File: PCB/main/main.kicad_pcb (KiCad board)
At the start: 2 copper layers, 4 parts, among them J1 Conn_01x33_Female, J2 Conn_01x33_Female, J3 Conn_01x33_Female, J4 Conn_01x33_Female

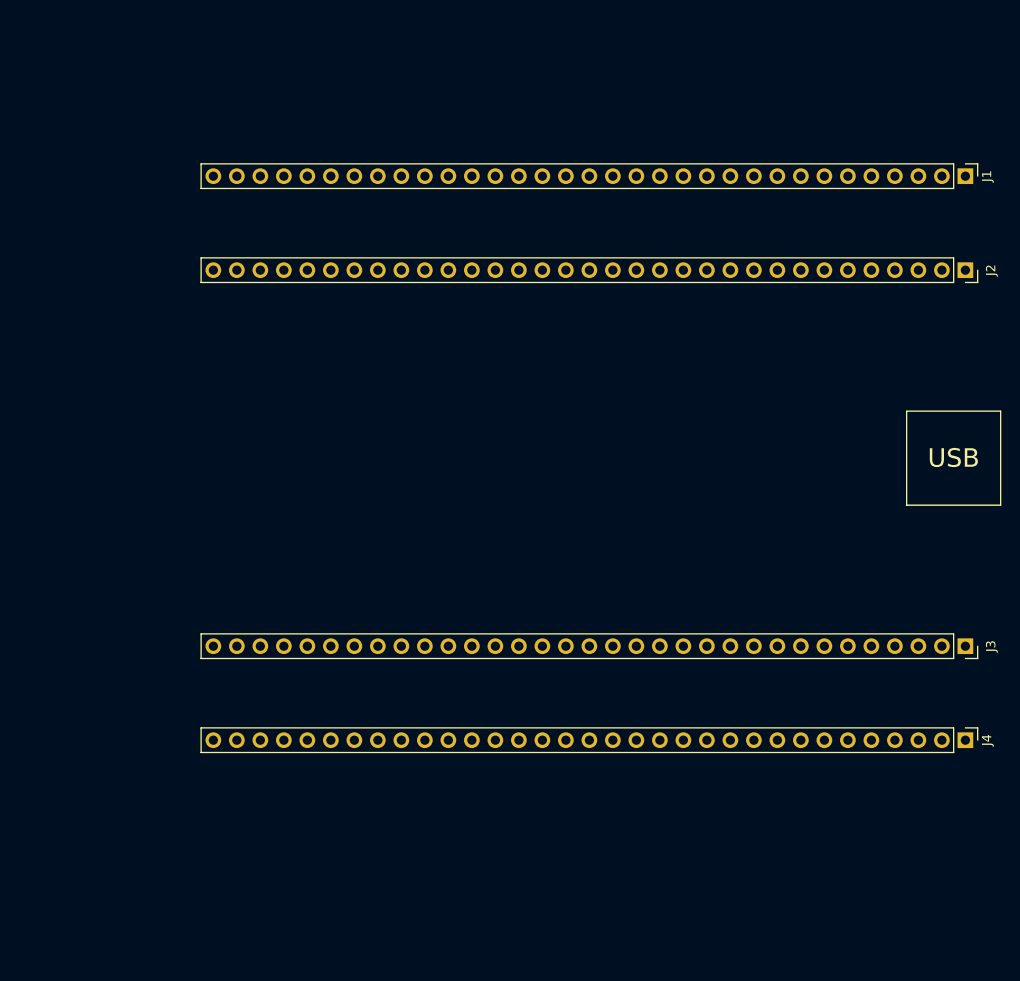
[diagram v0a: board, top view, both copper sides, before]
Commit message: NEW PCB ADDED
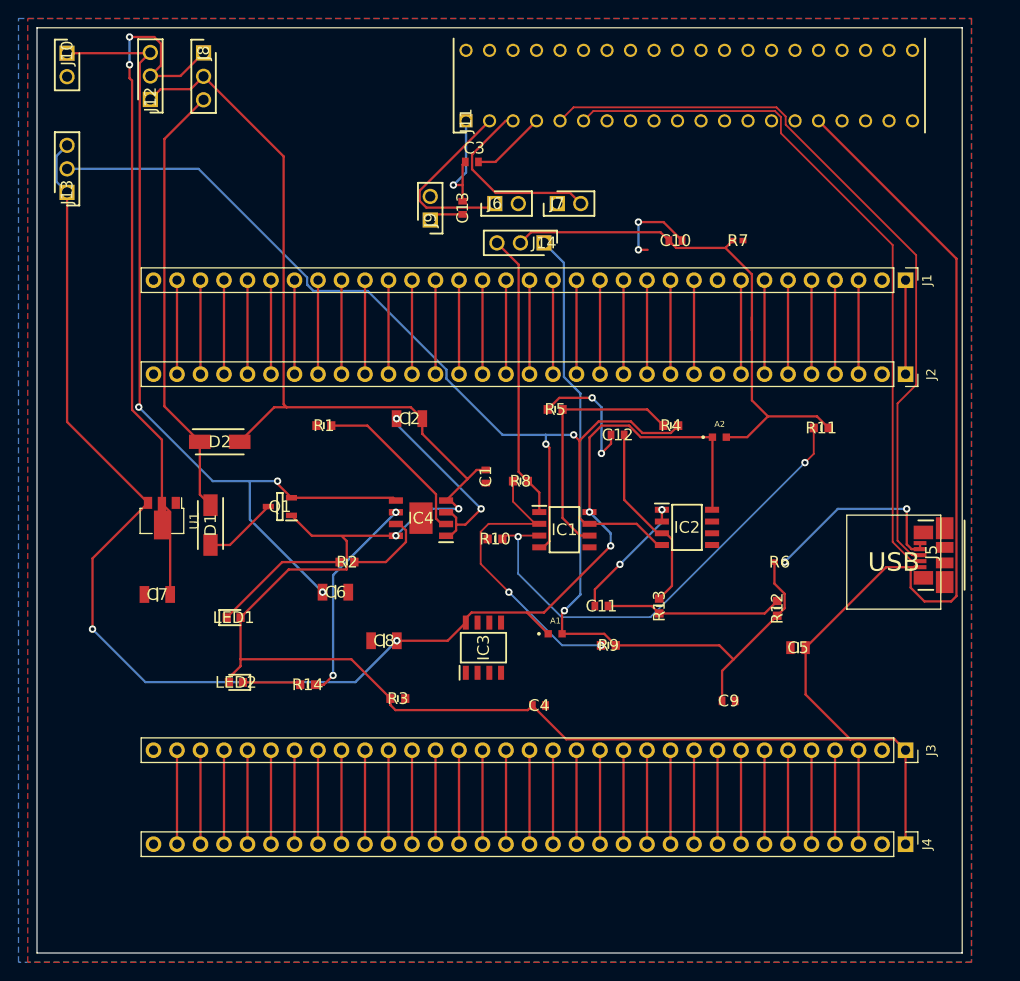
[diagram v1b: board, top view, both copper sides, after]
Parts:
- added A1: ALS-PT19-315C/L177/TR8, SamacSys_Parts:XDCR_ALS-PT19-315C_L177_TR8, F.Cu at (136.0, 115.5)
- added A2: ALS-PT19-315C/L177/TR8, SamacSys_Parts:XDCR_ALS-PT19-315C_L177_TR8, F.Cu at (153.8, 94.2)
- added C1: 10nF, SamacSys_Parts:CAPC1608X90N, F.Cu at (128.5, 98.5)
- added C10: CL10A105KB8NNNC, SamacSys_Parts:CAPC1608X90N, F.Cu at (149.0, 73.0)
- added C11: CL10A335KP8NNNC, SamacSys_Parts:CAPC1608X90N, F.Cu at (141.0, 112.5)
- added C12: CL10A335KP8NNNC, SamacSys_Parts:CAPC1608X90N, F.Cu at (142.8, 94.0)
- added C13: CC0603KRX7R9BB104, SamacSys_Parts:CAPC1608X90N, F.Cu at (126.0, 69.5)
- added C2: CL31A106KBHNNNE, SamacSys_Parts:CAPC3216X180N, F.Cu at (120.2, 92.2)
- added C3: 100nF, SamacSys_Parts:CAPC1608X90N, F.Cu at (127.0, 64.5)
- added C4: 100nF, SamacSys_Parts:CAPC1608X90N, F.Cu at (134.2, 123.2)
- added C5: CL21C101JBANNNC, SamacSys_Parts:CAPC2012X75N, F.Cu at (162.2, 117.0)
- added C6: CL31A106KBHNNNE, SamacSys_Parts:CAPC3216X180N, F.Cu at (112.2, 111.0)
- added C7: CL31A106KBHNNNE, SamacSys_Parts:CAPC3216X180N, F.Cu at (93.0, 111.2)
- added C8: CL31A106KBHNNNE, SamacSys_Parts:CAPC3216X180N, F.Cu at (117.5, 116.2)
- added C9: CL10A105KB8NNNC, SamacSys_Parts:CAPC1608X90N, F.Cu at (154.8, 122.8)
- added D1: SS14, SamacSys_Parts:DIOM5227X270N, F.Cu at (98.8, 103.8)
- added D2: SS14, SamacSys_Parts:DIOM5227X270N, F.Cu at (99.8, 94.8)
- added IC1: LM358DT, SamacSys_Parts:SOIC127P600X175-8N, F.Cu at (137.0, 104.2)
- added IC2: LM358DT, SamacSys_Parts:SOIC127P600X175-8N, F.Cu at (150.2, 104.0)
- added IC3: AT24C256C-SSHL-T, SamacSys_Parts:SOIC127P600X175-8N, F.Cu at (128.2, 117.0)
- added IC4: TP4056-42-ESOP8, SamacSys_Parts:SOIC127P600X175-9N, F.Cu at (121.5, 103.0)
- added J10: PZ254V-11-02P, SamacSys_Parts:HDRV2W64P0X254_1X2_508X250X873P, F.Cu at (83.2, 52.8)
- added J11: ICH-340-CTT, SamacSys_Parts:DIPS762W74P254L5080H338Q40N, F.Cu at (126.4, 60.1)
- added J12: MTP125-1103S1, SamacSys_Parts:HDRV3W64P0X254_1X3_762X250X885P, F.Cu at (92.2, 57.8)
- added J13: MTP125-1103S1, SamacSys_Parts:HDRV3W64P0X254_1X3_762X250X885P, F.Cu at (83.2, 67.8)
- added J14: MTP125-1103S1, SamacSys_Parts:HDRV3W64P0X254_1X3_762X250X885P, F.Cu at (134.8, 73.2)
- added J5: 47346-0001, SamacSys_Parts:47346-0001, F.Cu at (180.2, 107.0)
- added J6: PZ254V-11-02P, SamacSys_Parts:HDRV2W64P0X254_1X2_508X250X873P, F.Cu at (129.5, 69.0)
- added J7: PZ254V-11-02P, SamacSys_Parts:HDRV2W64P0X254_1X2_508X250X873P, F.Cu at (136.2, 69.0)
- added J8: MTP125-1103S1, SamacSys_Parts:HDRV3W64P0X254_1X3_762X250X885P, F.Cu at (98.0, 52.7)
- added J9: PZ254V-11-02P, SamacSys_Parts:HDRV2W64P0X254_1X2_508X250X873P, F.Cu at (122.5, 70.8)
- added LED1: 19-217_GHC-YR1S2_3T, SamacSys_Parts:LEDC1608X50N, F.Cu at (101.2, 113.8)
- added LED2: 19-217_GHC-YR1S2_3T, SamacSys_Parts:LEDC1608X50N, F.Cu at (101.5, 120.8)
- added Q1: AO3401A, SamacSys_Parts:SOT95P280X125-3N, F.Cu at (106.2, 101.8)
- added R1: 0603WAF1201T5E, SamacSys_Parts:RESC1608X55N, F.Cu at (111.0, 93.0)
- added R10: RC0603FR-071KL, SamacSys_Parts:RESC1608X55N, F.Cu at (129.5, 105.2)
- added R11: RC0603FR-071KL, SamacSys_Parts:RESC1608X55N, F.Cu at (164.8, 93.2)
- added R12: RC0603FR-071KL, SamacSys_Parts:RESC1608X55N, F.Cu at (160.0, 112.8)
- added R13: RC0603FR-071KL, SamacSys_Parts:RESC1608X55N, F.Cu at (147.2, 112.5)
- added R14: RC0603FR-071KL, SamacSys_Parts:RESC1608X55N, F.Cu at (109.2, 121.0)
- added R2: RC0603FR-071KL, SamacSys_Parts:RESC1608X55N, F.Cu at (113.5, 107.8)
- added R3: 10k, SamacSys_Parts:RESC1608X55N, F.Cu at (119.0, 122.5)
- added R4: RC0603FR-071KL, SamacSys_Parts:RESC1608X55N, F.Cu at (148.5, 93.0)
- added R5: RC0603FR-071KL, SamacSys_Parts:RESC1608X55N, F.Cu at (136.0, 91.2)
- added R6: AC0402FR-07536KL, SamacSys_Parts:RESC1005X37N, F.Cu at (160.2, 107.8)
- added R7: AC0402FR-07536KL, SamacSys_Parts:RESC1005X37N, F.Cu at (155.8, 73.0)
- added R8: RC0603FR-071KL, SamacSys_Parts:RESC1608X55N, F.Cu at (132.2, 99.0)
- added R9: RC0603FR-071KL, SamacSys_Parts:RESC1608X55N, F.Cu at (141.8, 116.8)
- added U1: HT75xx-1-SOT89, Package_TO_SOT_SMD:SOT-89-3, F.Cu at (93.5, 103.0)
- moved J3 13.0 mm to (173.9, 128.1)
- moved J4 13.0 mm to (173.9, 138.2)
- moved J1 13.0 mm to (173.9, 77.3)
- moved J2 13.0 mm to (173.9, 87.4)
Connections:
- net +5V renamed 5V USB
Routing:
- net 5V USB: track 0.00 -> 310.3 mm, vias 0 -> 2
- net +3v3: track 0.00 -> 162.2 mm, vias 0 -> 4
- net -3v3: track 0.00 -> 112.4 mm, vias 0 -> 2
- net BAT volt: track 0.00 -> 95.3 mm, vias 0 -> 3
- net Vout1: track 0.00 -> 82.6 mm, vias 0 -> 1
- net /Power/D+: track 0.00 -> 81.0 mm
- net GND: track 0.00 -> 79.3 mm, vias 0 -> 9
- net /Power/D-: track 0.00 -> 76.8 mm
- net LDO: track 0.00 -> 76.5 mm, vias 0 -> 2
- net Vout2: track 0.00 -> 58.5 mm
- net IN1+: track 0.00 -> 52.1 mm, vias 0 -> 2
- net Net-(D1-Pad1): track 0.00 -> 47.6 mm
- net IN1-: track 0.00 -> 32.9 mm, vias 0 -> 2
- net Vdiff: track 0.00 -> 31.0 mm
- net IN2-: track 0.00 -> 27.1 mm
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- added copper zone on B.Cu, net +3v3
- added copper zone on F.Cu, net GND
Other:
- board outline added: 100 x 100 mm
